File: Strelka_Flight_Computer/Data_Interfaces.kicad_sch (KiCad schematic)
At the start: 9 parts, among them J16 Conn_01x04, J6 USB_B_Micro, U8 MCP2551-I-SN, U8 USBLC6-2SC6

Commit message: Created BOM
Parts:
- U8: LCSC (none) -> C2687116; LCSC# C2687116 -> (none)
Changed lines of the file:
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@@
       (effects (font (size 1.27 1.27)) hide)
     )
-    (property "LCSC#" "C2687116" (at 146.05 69.215 90)
+    (property "LCSC" "C2687116" (at 146.05 69.215 90)
       (effects (font (size 1.27 1.27)) hide)
     )

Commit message: Added LCSC mpn to all relevent parts
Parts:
- C35: LCSC (none) -> C1525
- R51: LCSC (none) -> C11702
- R52: LCSC (none) -> C25079
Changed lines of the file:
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@@
+      (effects (font (size 1.27 1.27)) hide)
+    )
+    (property "LCSC" " C1525" (at 157.48 103.505 0)
       (effects (font (size 1.27 1.27)) hide)
     )
@@
     )
     (property "Datasheet" "~" (at 149.86 123.825 0)
+      (effects (font (size 1.27 1.27)) hide)
+    )
+    (property "LCSC" "C25079" (at 149.86 123.825 0)
       (effects (font (size 1.27 1.27)) hide)
     )
@@
       (effects (font (size 1.27 1.27)) hide)
     )
+    (property "LCSC" " C11702" (at 107.95 132.715 0)
+      (effects (font (size 1.27 1.27)) hide)
+    )

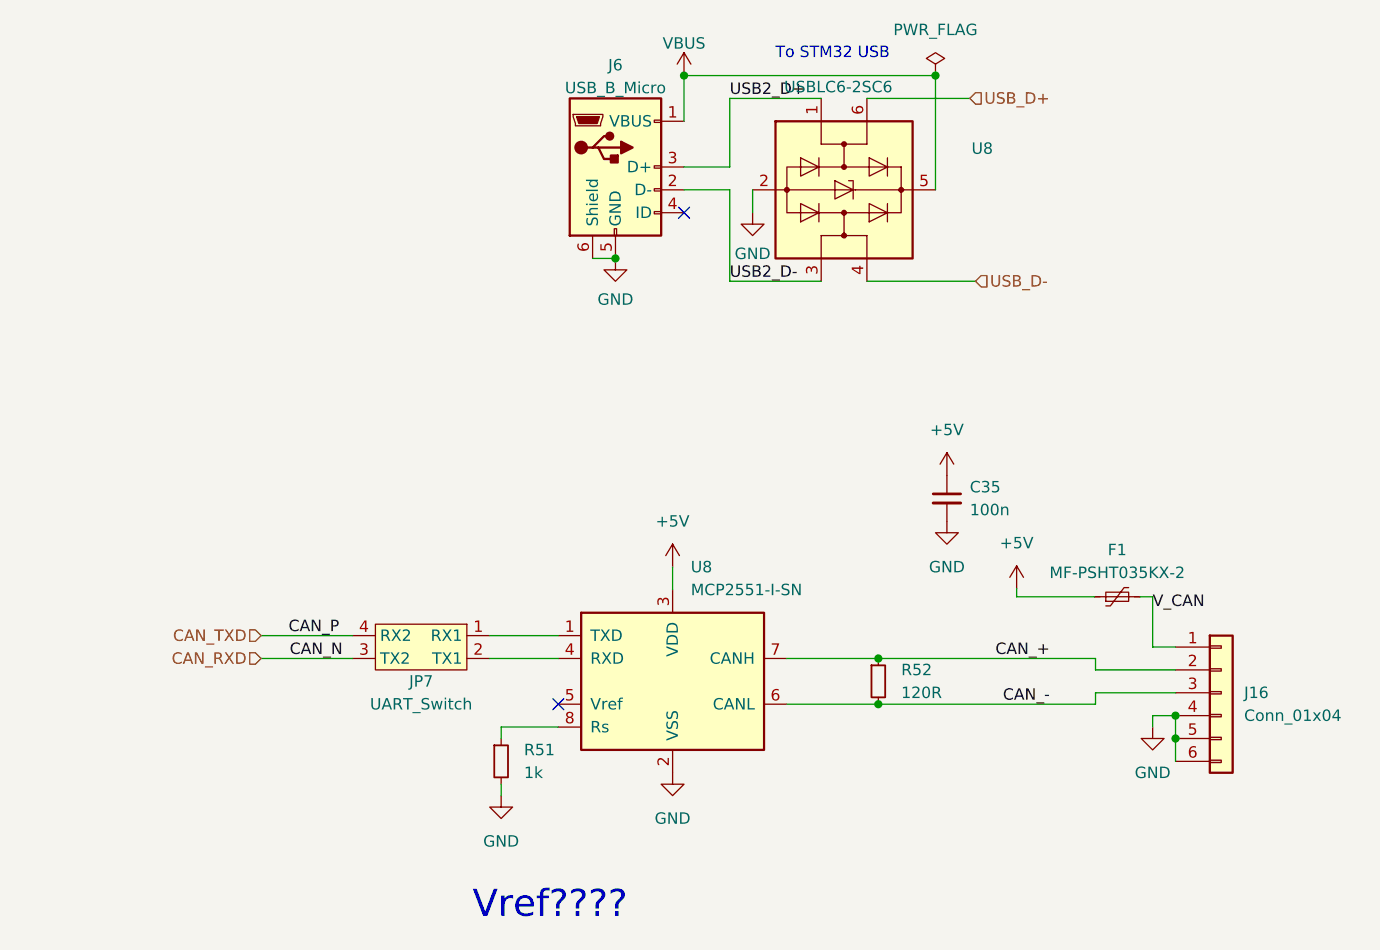
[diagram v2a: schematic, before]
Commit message: Finalised BOM and sent order:
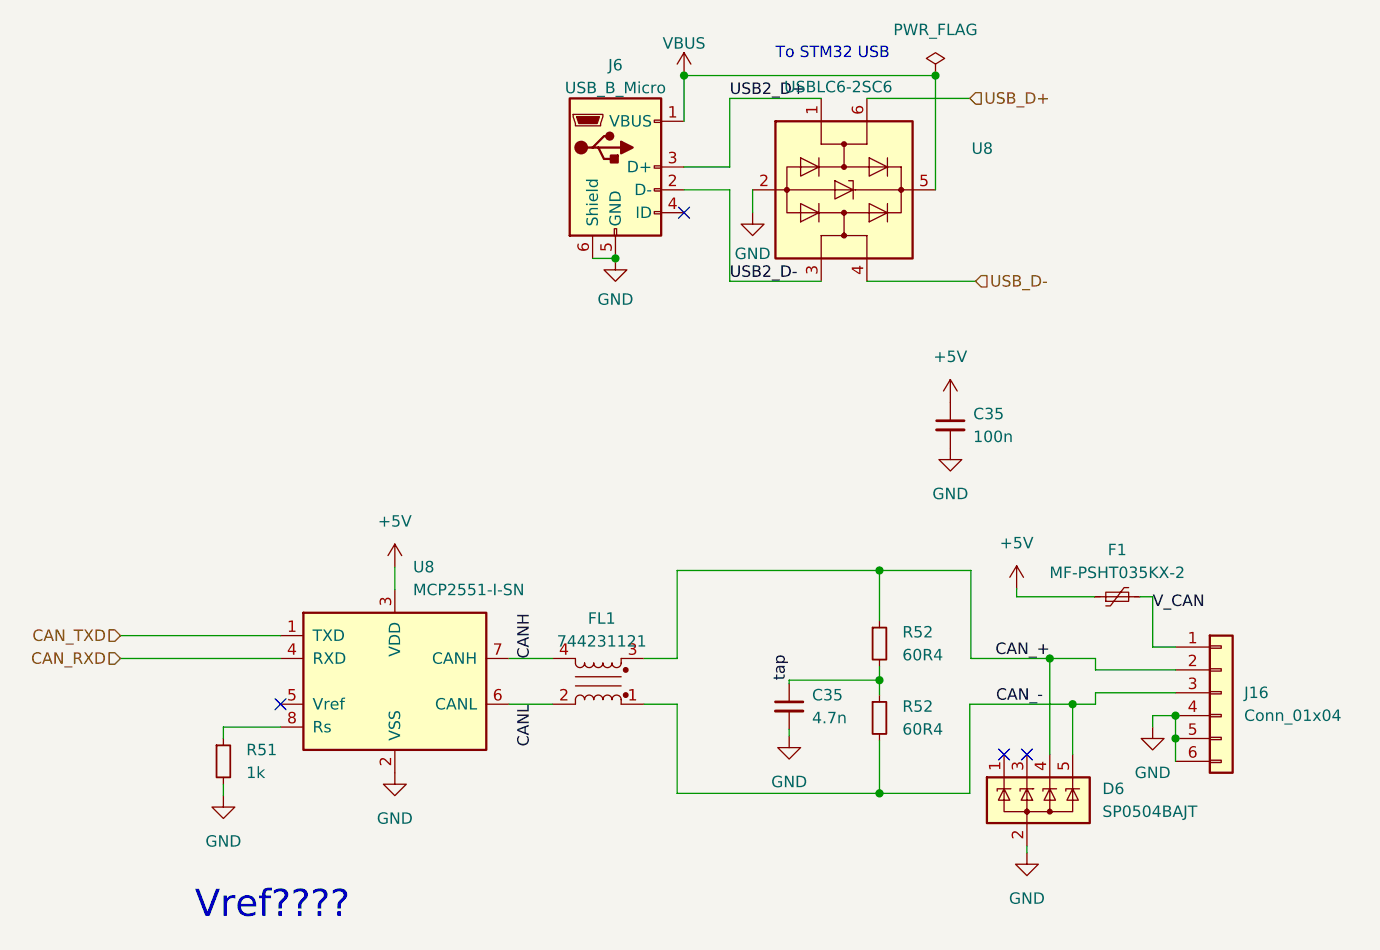
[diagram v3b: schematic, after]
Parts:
- removed JP7: UART_Switch, Footprints:UART_Switch, symbol UART_Switch:UART_Switch
- added C35: 4.7n, Capacitor_SMD:C_0603_1608Metric, symbol Device:C_Small
- added D6: SP0504BAJT, Package_TO_SOT_SMD:SOT-353_SC-70-5, symbol Power_Protection:SP0504BAJT
- added FL1: 744231121, Footprints:CHIP_31121_WRE, symbol Filter:Choke_Schaffner_RN102-0.3-02-12M
- added R52: 60R4, Resistor_SMD:R_0402_1005Metric, symbol Device:R_Small
- R52: value 120R -> 60R4; LCSC C25079 -> C241122
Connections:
- net CAN_+: now also D6.4 (K), FL1.3; no longer U8.7 (CANH)
- net CAN_-: now also D6.5 (K), FL1.1, R52.2; no longer R52.2, U8.6 (CANL)
- net CAN_RXD: now also U8.4 (RXD)
- net CAN_TXD: now also U8.1 (TXD)
- net GND: now also C35.2, D6.2 (A)
- new net CANH: FL1.4, U8.7 (CANH)
- new net CANL: FL1.2, U8.6 (CANL)
- new net tap: C35.1, R52.1, R52.2
- no-connect marks 2 -> 4
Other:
- moved on the sheet: C35, R51, R52, U8
